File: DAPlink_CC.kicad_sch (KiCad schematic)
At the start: 70 parts

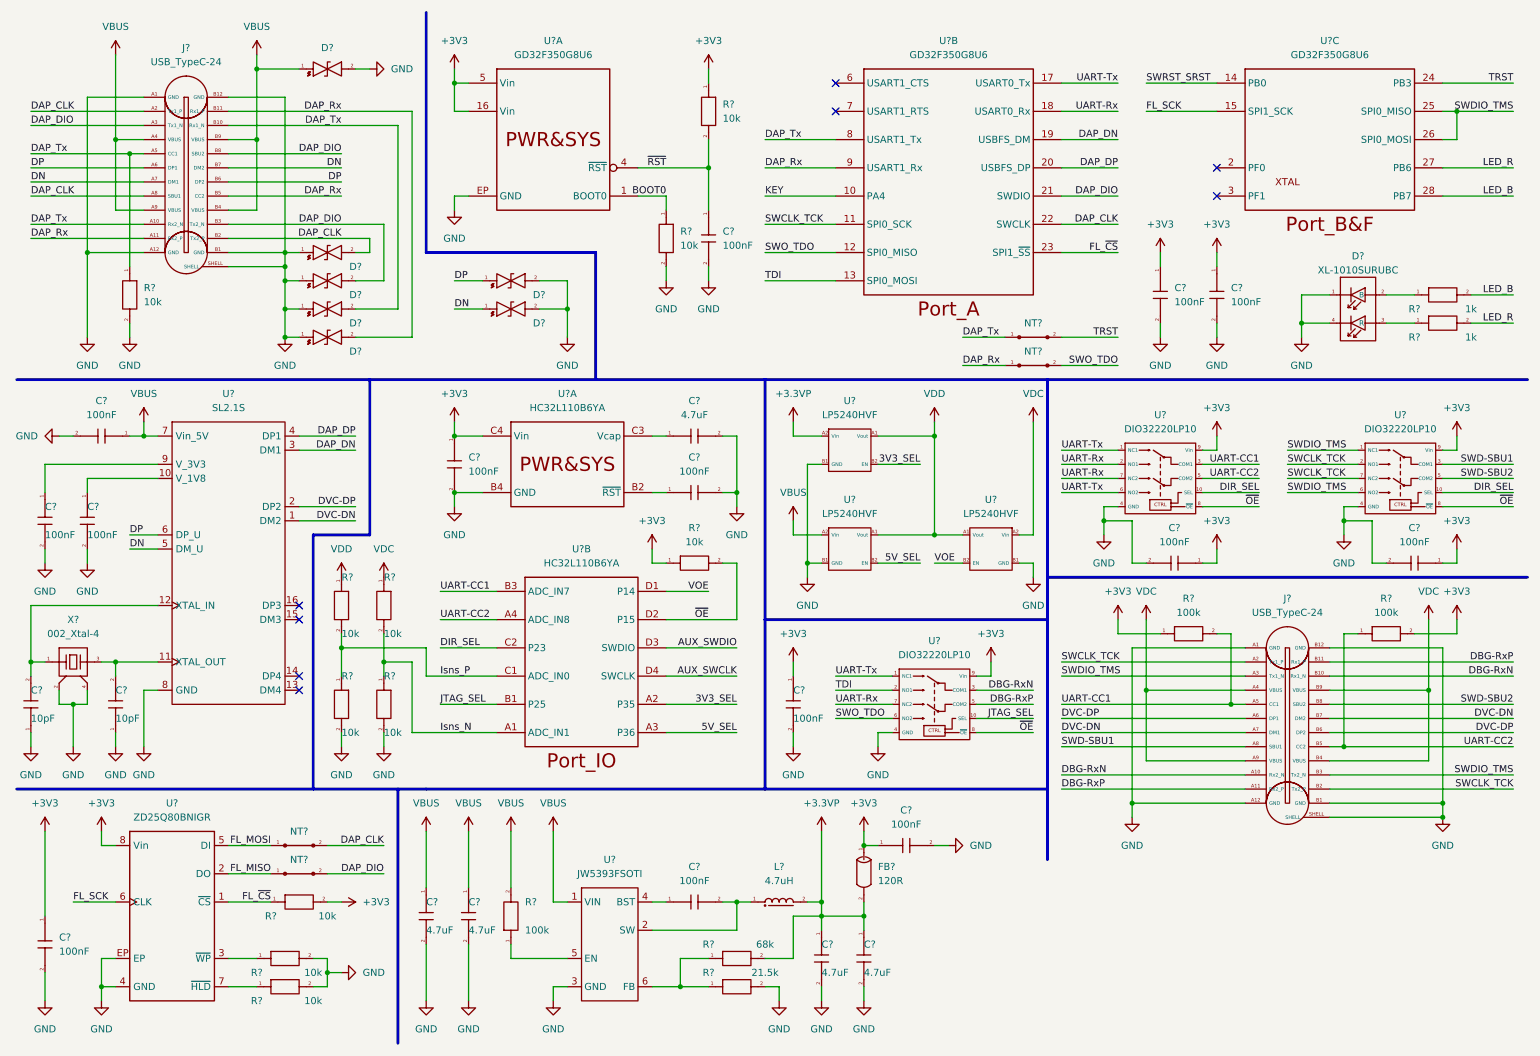
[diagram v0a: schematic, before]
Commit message: Update schematics
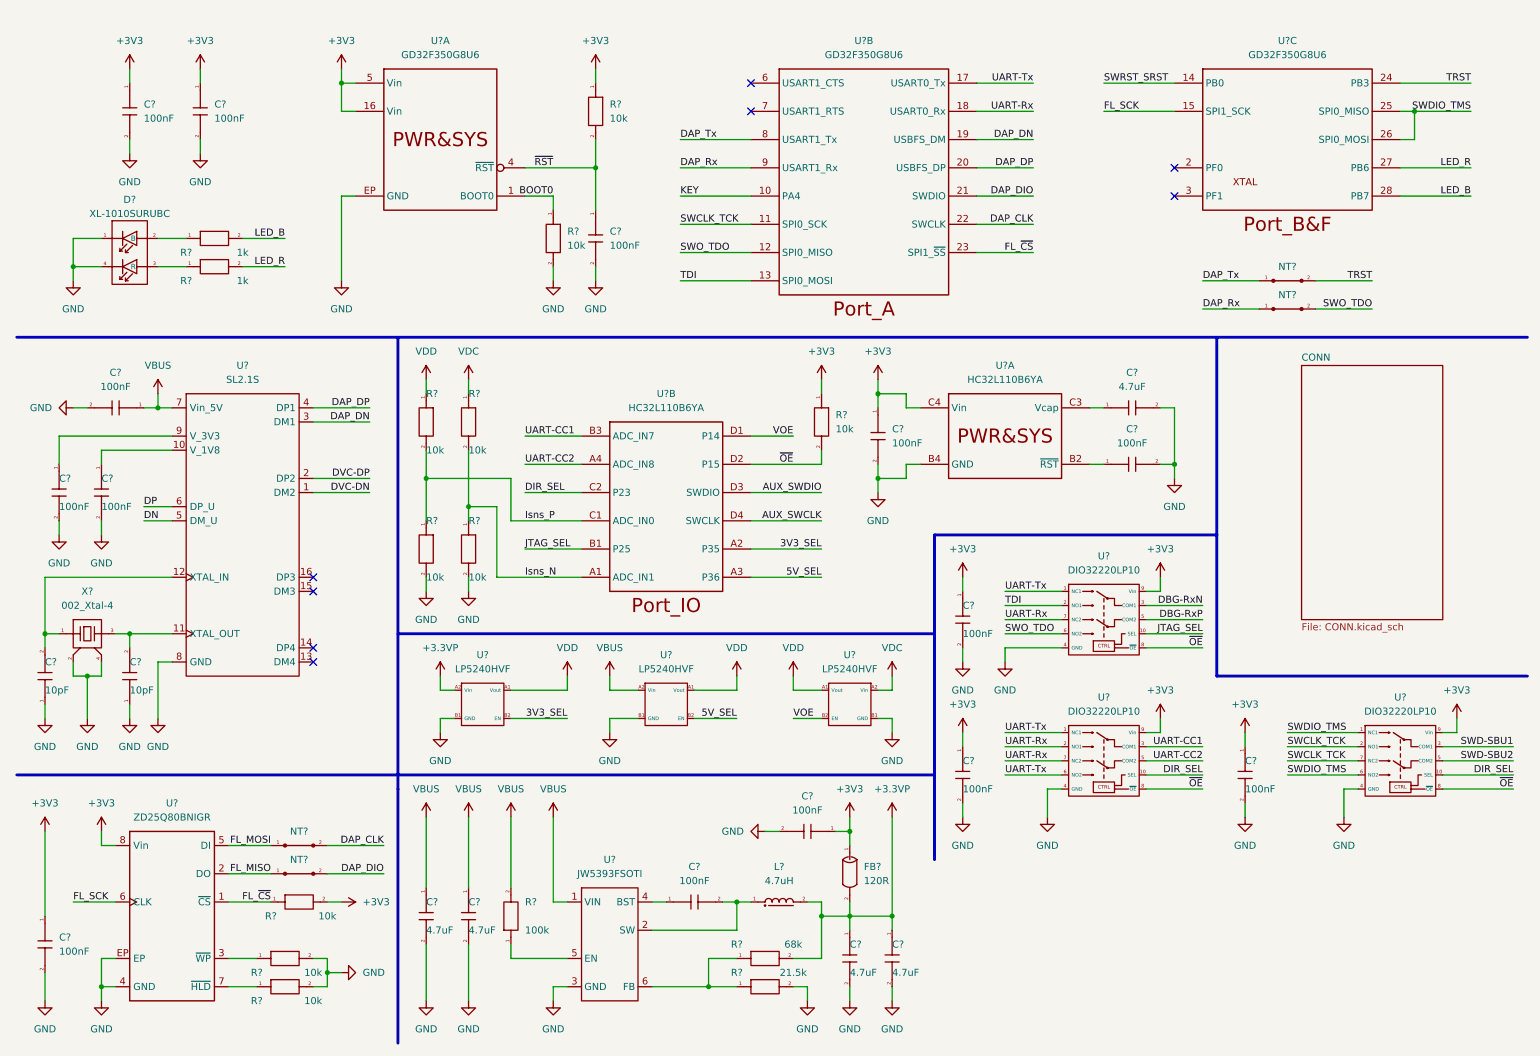
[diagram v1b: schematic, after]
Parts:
- removed C? (x3): 100nF, 001_GN_RCL_SMD:C0201(0603M), symbol 001_Basic_PassiveComponents:101_Capacitor
- removed D? (x7): LESD11LL5.0CT5G, 002_GN_TWO-PIN_PLASTIC_SMD:SOD-123, symbol 002_Basic_SingleSemiconductor:007_Diode_ESD_Bi
- removed J? (x2): USB_TypeC-24, symbol 306_Link_USB-Connector:USB_TypeC-24
- removed R?: 10k, 001_GN_RCL_SMD:R0201(0603M), symbol 001_Basic_PassiveComponents:001_Resistor
- removed R? (x2): 100k, 001_GN_RCL_SMD:R0201(0603M), symbol 001_Basic_PassiveComponents:001_Resistor
- removed U? (x3): LP5240HVF, 104_SP_SMALL_SMD:CSP-4_S7575, symbol 110_IntegratedCircuit_Interface:LP5240HVF
- removed U? (x3): DIO32220LP10, 003_GN_SMALL-SEMI_SMD:QFN-10_1814, symbol 110_IntegratedCircuit_Interface:DIO32220LP10
- added C? (x3): 100nF, 001_GN_RCL_SMD:C0201(0603M), symbol 001_Basic_PassiveComponents:101_Capacitor
- added U? (x3): LP5240HVF, 104_SP_SMALL_SMD:CSP-4_S7575, symbol 110_IntegratedCircuit_Interface:LP5240HVF
- added U? (x3): DIO32220LP10, 003_GN_SMALL-SEMI_SMD:QFN-10_1814, symbol 110_IntegratedCircuit_Interface:DIO32220LP10
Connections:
- net +3.3VP: now also U?.A2 (Vin)
- net +3V3: now also C?.1, C?.1, C?.1, U?.9 (Vin), U?.9 (Vin), U?.9 (Vin)
- net 3V3_SEL: now also U?.B2 (EN)
- net 5V_SEL: now also U?.B2 (EN)
- net DBG-RxN: now also U?.3 (COM1)
- net DBG-RxP: now also U?.5 (COM2)
- net DIR_SEL: now also U?.10 (SEL), U?.10 (SEL)
- net GND: now also C?.2, C?.2, C?.2, U?.4 (GND), U?.4 (GND), U?.4 (GND), U?.B1 (GND), U?.B1 (GND), U?.B1 (GND)
- net JTAG_SEL: now also U?.10 (SEL)
- net SWCLK_TCK: now also U?.2 (NO1), U?.7 (NC2)
- net SWD-SBU1: now also U?.3 (COM1)
- net SWD-SBU2: now also U?.5 (COM2)
- net SWDIO_TMS: now also U?.1 (NC1), U?.6 (NO2)
- net SWO_TDO: now also U?.6 (NO2)
- net TDI: now also U?.2 (NO1)
- net UART-CC1: now also U?.3 (COM1)
- net UART-CC2: now also U?.5 (COM2)
- net UART-Rx: now also U?.2 (NO1), U?.7 (NC2), U?.7 (NC2)
- net UART-Tx: now also U?.1 (NC1), U?.1 (NC1), U?.6 (NO2)
- net VBUS: now also U?.A2 (Vin)
- net VDC: now also U?.A2 (Vin)
- net VDD: now also U?.A1 (Vout), U?.A1 (Vout), U?.A1 (Vout)
- net VOE: now also U?.B2 (EN)
- net ~{OE}: now also U?.8 (~{OE}), U?.8 (~{OE}), U?.8 (~{OE})
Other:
- added sheet CONN (CONN.kicad_sch)
- moved on the sheet: C?, D?, FB?, NT?, R?, U?, U?A, U?B, U?C, X?
